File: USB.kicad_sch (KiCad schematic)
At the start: 1 part, among them J1 USB_A

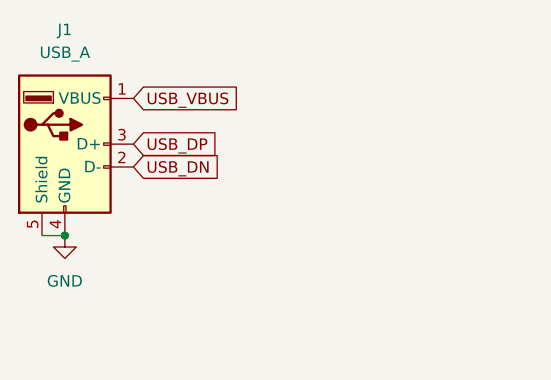
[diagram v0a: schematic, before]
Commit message: progress
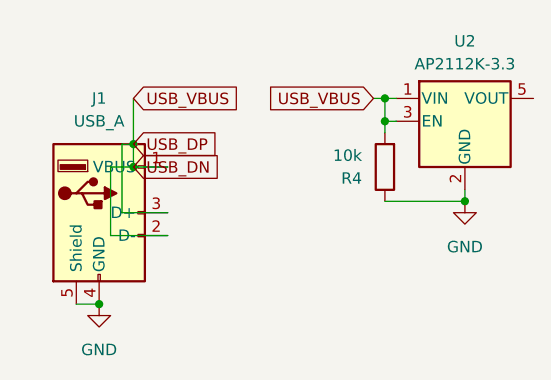
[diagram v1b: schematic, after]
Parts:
- added R4: 10k, symbol Device:R
- added U2: AP2112K-3.3, Package_TO_SOT_SMD:SOT-23-5, symbol Regulator_Linear:AP2112K-3.3
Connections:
- net USB_DP is gone; now on net USB_DN: J1.3 (D+)
- net USB_VBUS is gone; now on net USB_DN: J1.1 (VBUS)
- net GND: now also R4.1, U2.2 (GND)
- net USB_DN: now also R4.2, U2.1 (VIN), U2.3 (EN)
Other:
- moved on the sheet: J1

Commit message: progress
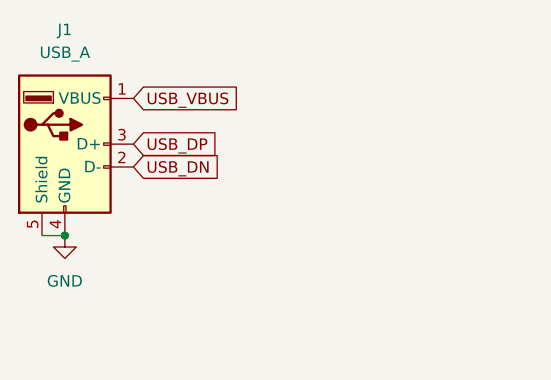
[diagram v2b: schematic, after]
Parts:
- removed R4: 10k, symbol Device:R
- removed U2: AP2112K-3.3, Package_TO_SOT_SMD:SOT-23-5, symbol Regulator_Linear:AP2112K-3.3
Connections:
- net USB_DN: no longer J1.1 (VBUS), J1.3 (D+)
- new net USB_DP: J1.3 (D+)
- new net USB_VBUS: J1.1 (VBUS)
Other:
- moved on the sheet: J1

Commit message: progress
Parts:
- J1: footprint (none) -> Connector_USB:USB_A_Receptacle_GCT_USB1046
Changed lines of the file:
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@@
 			)
 		)
-		(property "Footprint" ""
+		(property "Footprint" "Connector_USB:USB_A_Receptacle_GCT_USB1046"
 			(at 29.21 34.29 0)
 			(effects
